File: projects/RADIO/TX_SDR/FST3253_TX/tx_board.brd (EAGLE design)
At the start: 100 x 80 mm, 24 parts, among them IC2 NE5532N, IC3 NE5532N

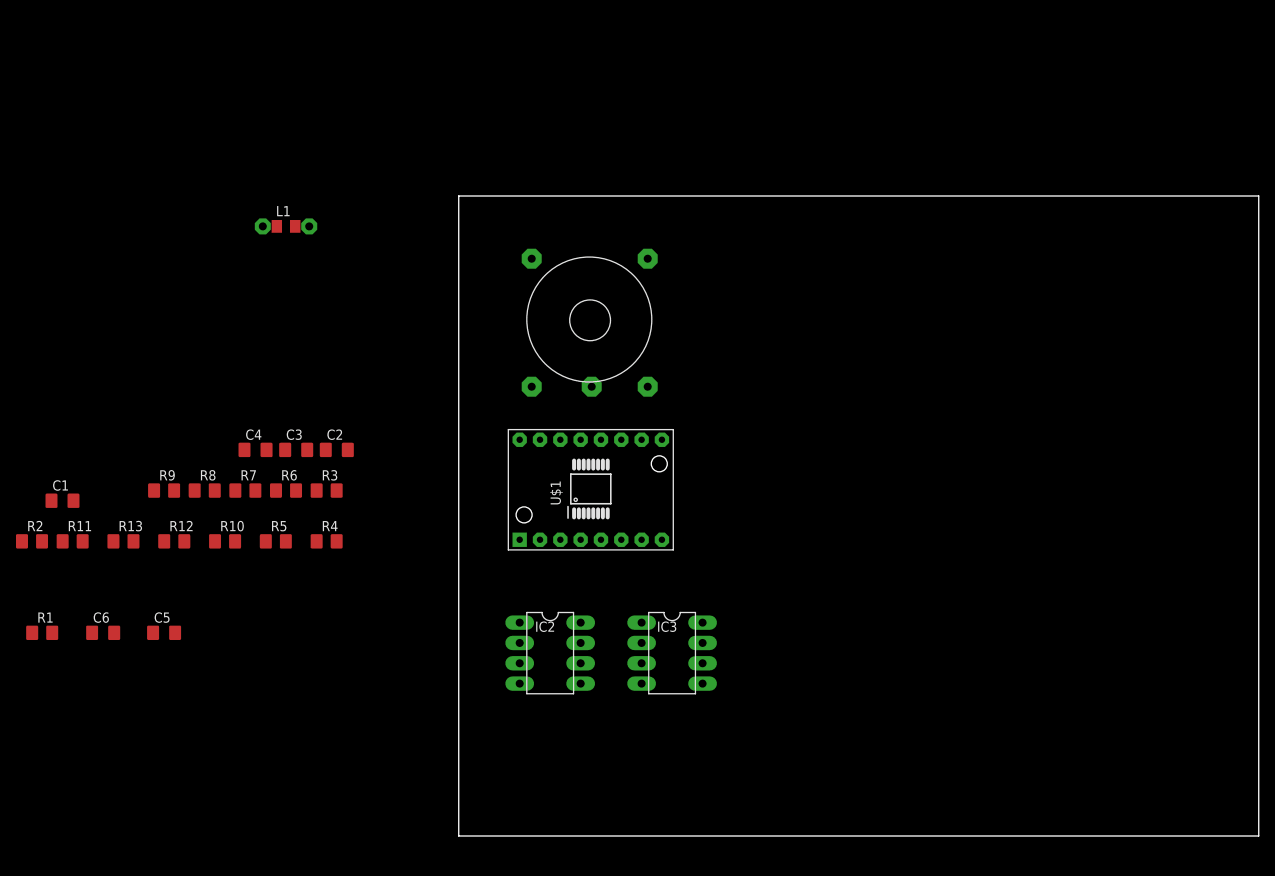
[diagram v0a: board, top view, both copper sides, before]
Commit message: Update
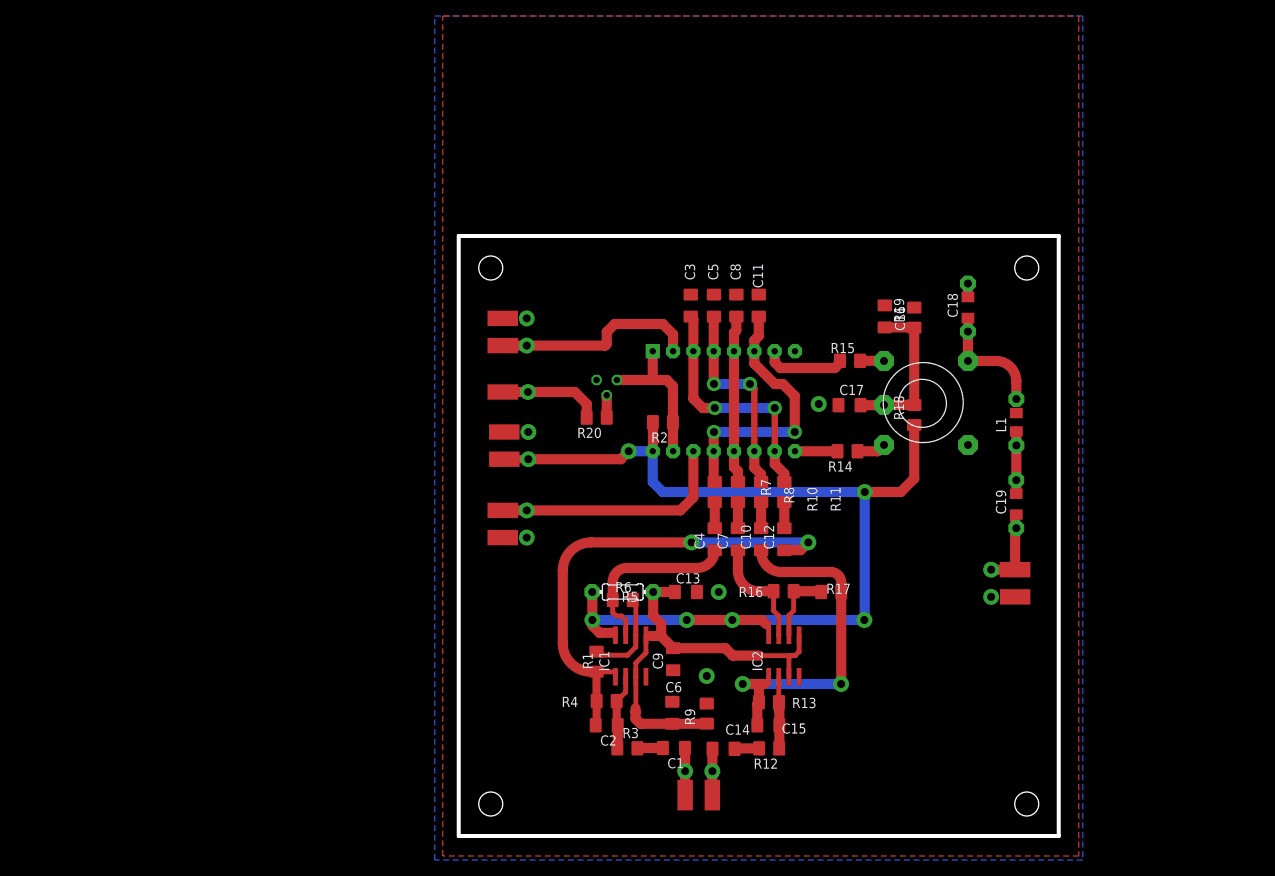
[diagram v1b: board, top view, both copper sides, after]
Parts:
- removed IC3: NE5532N, linear:DIL08
- added 5VDC, CLK1, CLK2, LINE_OUNT_IN, RF_OUT: 2X_SMD_PTH_PIN, mylib:2X_SMD_PTH
- added C10, C12, C14, C7: 10uF, mylib:C0805
- added C11, C8: 0.022uF, mylib:C0805
- added C13: 100nF, mylib:C0805
- added C15: 100pF, mylib:C0805
- added C16, C17: (no value), mylib:C0805
- added C18, C19: (no value), mylib:C0805K
- added C9: 4.7uF, mylib:C0805
- added IC1: NE5532D, linear:SO08
- added Q1: 2N3904, transistor-small-signal:TO92D
- added R14, R15: 50k, mylib:R0805W
- added R16, R17: 10k, mylib:R0805W
- added R18: 3.3k, mylib:R0805W
- added R19: 2.2k, mylib:R0805W
- added R20: 22k, mylib:R0805W
- added TX_DISABLE: SMD_PTH_PIN, mylib:SMD_PTH_PIN
- C1, C4: value (none) -> 10uF
- C2: value (none) -> 100pF
- C3: value (none) -> 0.022uF
- C5: value 100pF -> 0.022uF
- C6: value 100pF -> 100nF
- IC2: value NE5532N -> NE5532D; device linear:DIL08 -> linear:SO08
- R1: value 4.99k -> 10k
- R10, R11, R7, R8: value 10k -> 50k
- R2: value 50k -> 4.99k
- R3: value 50k -> 10k
- R4: value 2.2k -> 10k
- R5: value 3.3k -> 10k
- R6: value 10k -> 2.2k; device mylib:R0805W -> rcl:0204/7
- R9: value 10k -> 2.2k
- moved L1 94.5 mm to (69.7, 51.7), turned to 90 degrees
- moved R11 89.2 mm to (40.7, 43.0), turned to 270 degrees
- moved R13 83.2 mm to (38.8, 16.7)
- moved C1 82.4 mm to (26.9, 11.0), turned to 180 degrees
- moved R2 80.3 mm to (25.5, 51.7), turned to 180 degrees
- moved C5 80.0 mm to (31.9, 66.3), turned to 270 degrees
- moved R12 78.7 mm to (38.8, 10.9), turned to 180 degrees
- moved R9 73.3 mm to (31.0, 15.3), turned to 270 degrees
- moved C6 71.8 mm to (26.7, 15.4), turned to 270 degrees
- moved R1 69.4 mm to (17.2, 21.8), turned to 270 degrees
- moved R10 67.3 mm to (37.8, 43.0), turned to 270 degrees
- moved R8 66.7 mm to (34.9, 43.0), turned to 270 degrees
- moved TR1 58.9 mm to (65.2, 60.9), turned to 180 degrees
- moved R7 58.7 mm to (32.0, 43.0), turned to 270 degrees
- moved C4 58.5 mm to (32.0, 37.1), turned to 90 degrees
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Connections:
- removed net V+: IC2.8, IC3.8
- removed net V-: IC2.4, IC3.4
- new net N$18: C19.1, C19.P$1, RF_OUT.P$2, RF_OUT.T$2
- new net N$19: C1.1, LINE_OUNT_IN.P$1, LINE_OUNT_IN.T$1
- new net N$20: C14.1, LINE_OUNT_IN.P$2, LINE_OUNT_IN.T$2
- new net N$22: C14.2, R12.2
- new net N$23: C1.2, R3.2
- new net N$24: R20.2, TX_DISABLE.P$1, TX_DISABLE.P$2
- new net N$25: C12.2, R11.2
- new net N$26: C10.2, R10.2
- new net N$27: C7.2, R8.2
- new net N$29: C13.1, C6.2, C9.2, IC1.3, IC1.5, IC2.3, IC2.5, R6.1, R9.2
- net 0: now also C3.2, R11.1
- net 180: now also C11.2, R7.1
- net 270: now also C8.2, R8.1, U$1.P$12
- net 5V: now also 5VDC.P$2, 5VDC.T$2, IC1.8, IC2.8, R18.1, R2.2, R6.2; no longer R1.2, R5.1
- net 90: now also C5.2, R10.1
- net CLK0: now also CLK1.P$1, CLK1.T$1
- net CLK1: now also CLK2.P$2, CLK2.T$2
- net GND: now also 5VDC.P$1, 5VDC.T$1, C11.1, C13.2, C16.1, C17.1, C18.2, C18.P$2, C3.1, C5.1, C6.1, C8.1, C9.1, CLK1.P$2, CLK1.T$2, CLK2.P$1, CLK2.T$1, IC1.4, IC2.4, Q1.E, R19.2, R9.1, RF_OUT.P$1, RF_OUT.T$1; no longer C1.1, C2.1, C3.2, R4.2
- net N$1: now also Q1.C, R2.1; no longer R1.1
- net N$10: now also C12.1, C2.2, IC1.1, R1.2, R4.1; no longer C5.2, IC2.1, R12.1, R7.2
- net N$11: now also IC1.6, R1.1, R5.2; no longer IC2.6, R10.2, R7.1
- net N$12: now also C15.1, IC2.2, R12.1; no longer C6.1, IC3.2, R8.1
- net N$13: now also C10.1, C15.2, IC2.1, R17.2; no longer C6.2, IC3.1, R9.2
- net N$14: now also IC2.6, R16.2, R17.1; no longer IC3.6, R11.2, R9.1
- net N$15: now also C4.1, IC1.7, R5.1; no longer IC2.7, R10.1
- net N$16: now also C7.1, IC2.7, R16.1; no longer IC3.7, R11.1
- net N$17: now also C4.2, R7.2; no longer IC3.3, IC3.5
- net N$2: now also R15.2; no longer R2.2
- net N$21: now also Q1.B, R20.1; no longer U$1.P$12
- net N$3: now also R14.2; no longer R3.2
- net N$4: now also R14.1; no longer R3.1
- net N$5: now also R15.1; no longer R2.1
- net N$6: now also C16.2, C17.2, R18.2, R19.1; no longer C1.2, C2.2, R4.1, R5.2
- net N$7: now also C2.1, IC1.2, R3.1, R4.2; no longer C5.1, IC2.2, R12.2, R6.1
- net N$8: now also C18.1, C18.P$1; no longer C3.1
- net N$9: now also C19.2, C19.P$2; no longer C4.2
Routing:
- net 5V: track 0.00 -> 130.6 mm, vias 0 -> 6
- net N$10: track 0.00 -> 60.1 mm, vias 0 -> 2
- net N$29: track 0.00 -> 54.6 mm
- net N$13: track 0.00 -> 46.2 mm, vias 0 -> 2
- net 180: track 0.00 -> 33.9 mm, vias 0 -> 2
- net 0: track 0.00 -> 31.3 mm, vias 0 -> 2
- net CLK0: track 0.00 -> 30.3 mm
- net CLK1: track 0.00 -> 25.9 mm
- net 90: track 0.00 -> 25.8 mm, vias 0 -> 2
- net N$15: track 0.00 -> 22.1 mm
- net 270: track 0.00 -> 21.0 mm
- net N$6: track 0.00 -> 20.1 mm
- net N$1: track 0.00 -> 19.2 mm
- net N$8: track 0.00 -> 14.7 mm
- net N$16: track 0.00 -> 13.9 mm
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- added copper zone on layer 1, net GND
- added copper zone on layer 16, net GND
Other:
- board size 100 x 80 mm -> 75 x 75 mm
